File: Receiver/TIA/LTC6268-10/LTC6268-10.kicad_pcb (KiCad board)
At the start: 4 copper layers, 30 x 40 mm, 28 parts, among them J1 IN, J2 Vout, J3 TEST, J4 OUT, U1 LTC6268-10-SOT23

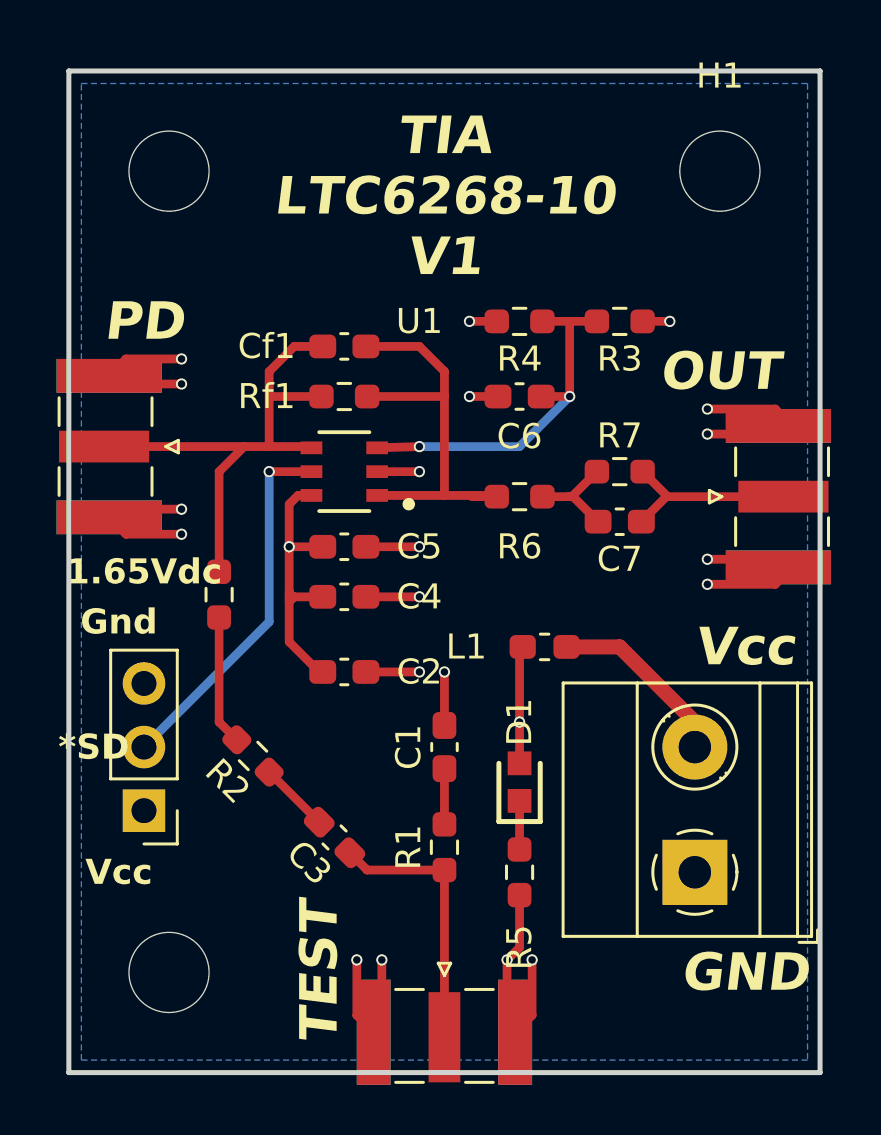
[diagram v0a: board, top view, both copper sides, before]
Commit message: LTC6268-10 first version
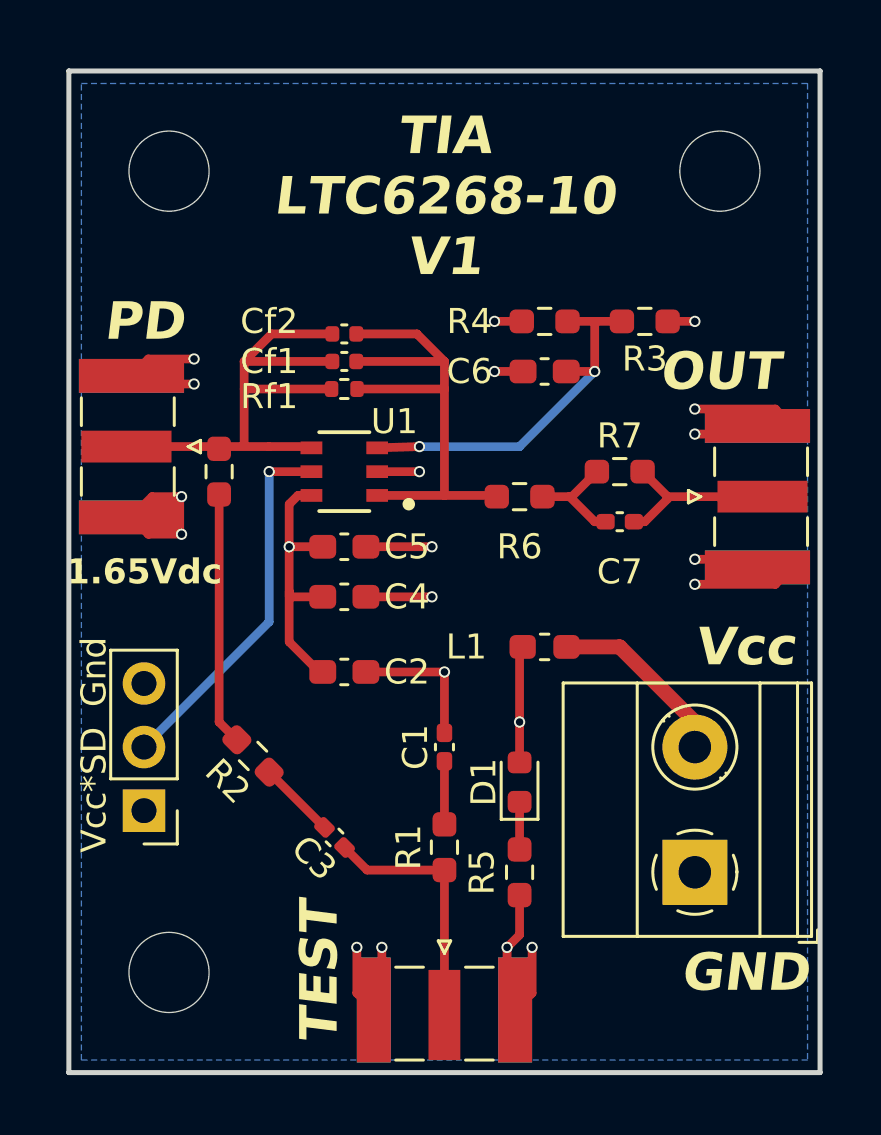
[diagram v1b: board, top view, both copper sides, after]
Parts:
- added Cf2: .5pF, Capacitor_SMD:C_0402_1005Metric, F.Cu at (117.9, 63.5)
- C1, C3, C7: value 1uF -> .1uF; footprint Capacitor_SMD:C_0603_1608Metric_Pad1.08x0.95mm_HandSolder -> Capacitor_SMD:C_0402_1005Metric_Pad0.74x0.62mm_HandSolder
- Cf1: value 10uF -> .2pF; footprint Capacitor_SMD:C_0603_1608Metric_Pad1.08x0.95mm_HandSolder -> Capacitor_SMD:C_0402_1005Metric
- D1: value 150060VS75000 -> Green Led; footprint LumiCom_TIA:LEDC1608X80N -> LED_SMD:LED_0603_1608Metric
- L1: value BLM18BA100SN1D -> Ferrite Beads 220 OHM
- R1, R6: value 50 -> 49.9
- R3, R4: value 20k -> 10k
- Rf1: value 10K -> 3k; footprint Resistor_SMD:R_0603_1608Metric_Pad0.98x0.95mm_HandSolder -> Resistor_SMD:R_0402_1005Metric
- U1: value LTC6268-10-SOT23 -> LTC6268-10
- moved JP1 4.91 mm to (112.9, 69.0)
- moved C6 1.41 mm to (125.9, 65.0)
- moved R3 1.00 mm to (129.9, 63.0)
- moved R4 1.00 mm to (125.9, 63.0)
- moved J1 0.89 mm to (109.4, 68.0)
- moved J3 0.89 mm to (121.9, 90.5)
- moved J4 0.84 mm to (134.4, 70.0)
- moved Cf1 0.60 mm to (117.9, 64.6)
- moved Rf1 0.30 mm to (117.9, 65.7)
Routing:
- net Net-(JP1-A): track 5.18 -> 10.1 mm
- net Net-(U1-OUT): track 17.4 -> 21.1 mm
- net Net-(J1-In): track 19.8 -> 21.1 mm
- net GND: track 54.4 -> 54.0 mm, vias 19 -> 18
